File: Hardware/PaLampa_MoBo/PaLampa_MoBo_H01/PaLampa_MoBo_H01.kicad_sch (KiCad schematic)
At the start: 47 parts, among them J1 Conn_01x03_Male, J9 Conn_01x05_Male, Q1 2N7002, Q4 2N7002, SW1 SW_SPST, SW2 SW_SPST, SW3 SW_SPST, U1 ESP32-WROOM-32D, U2 DS18B20, U3 OLED_I2C

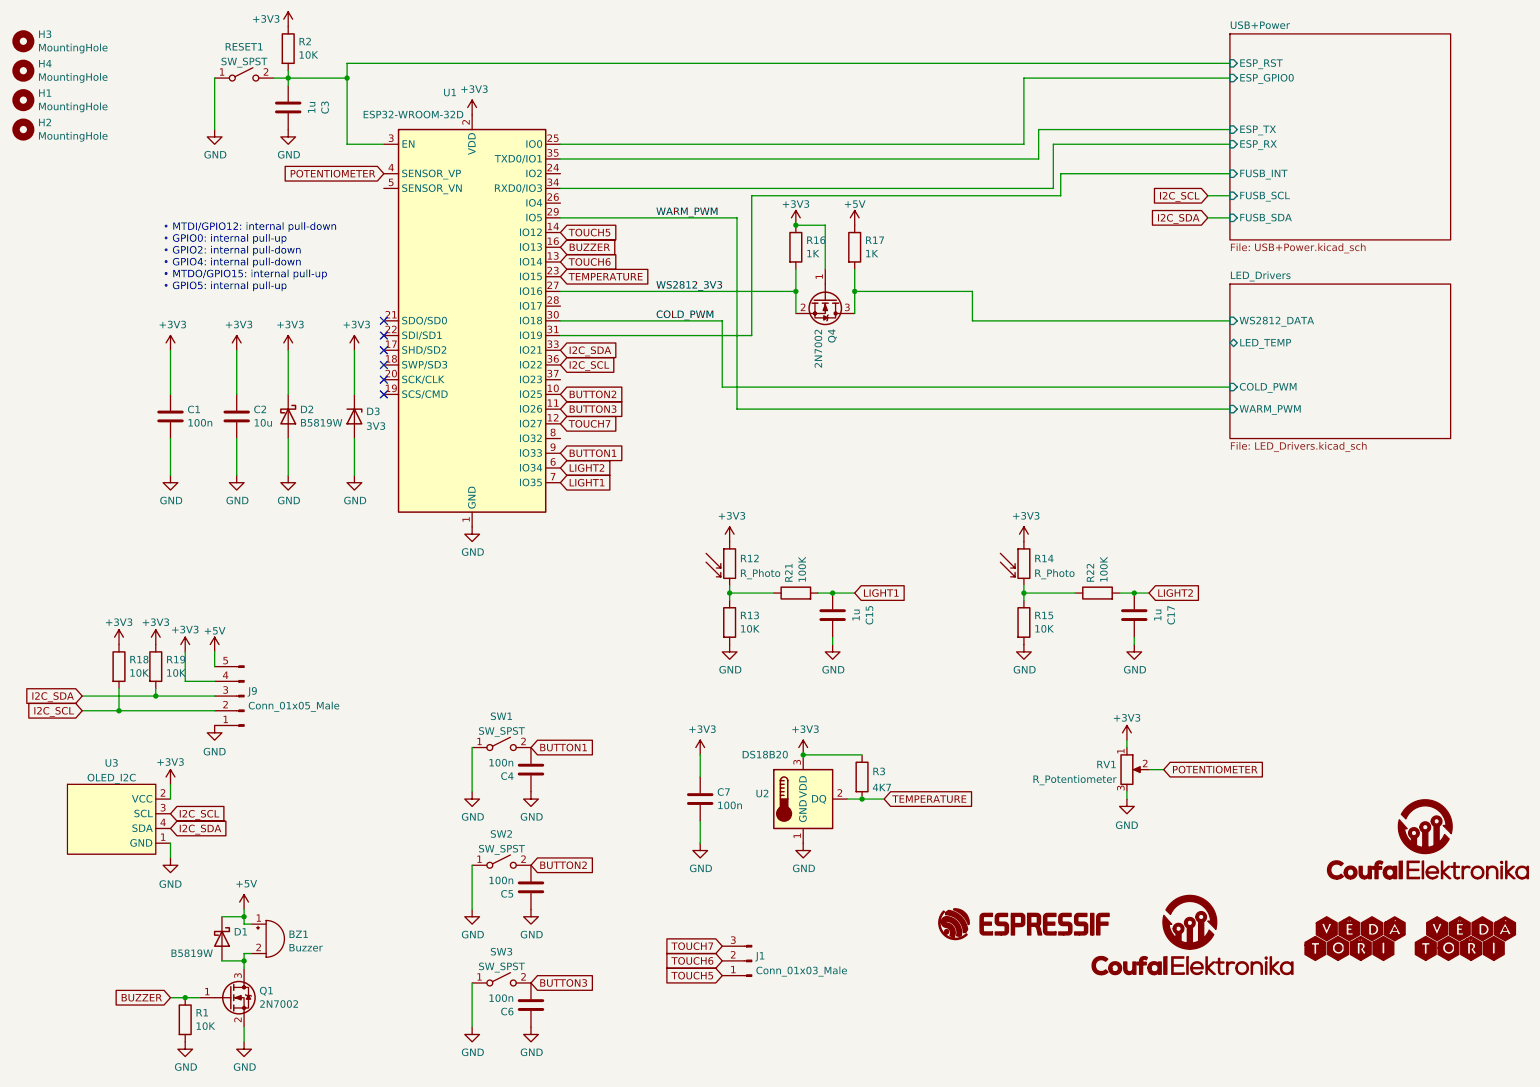
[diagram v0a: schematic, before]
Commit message: H01 update
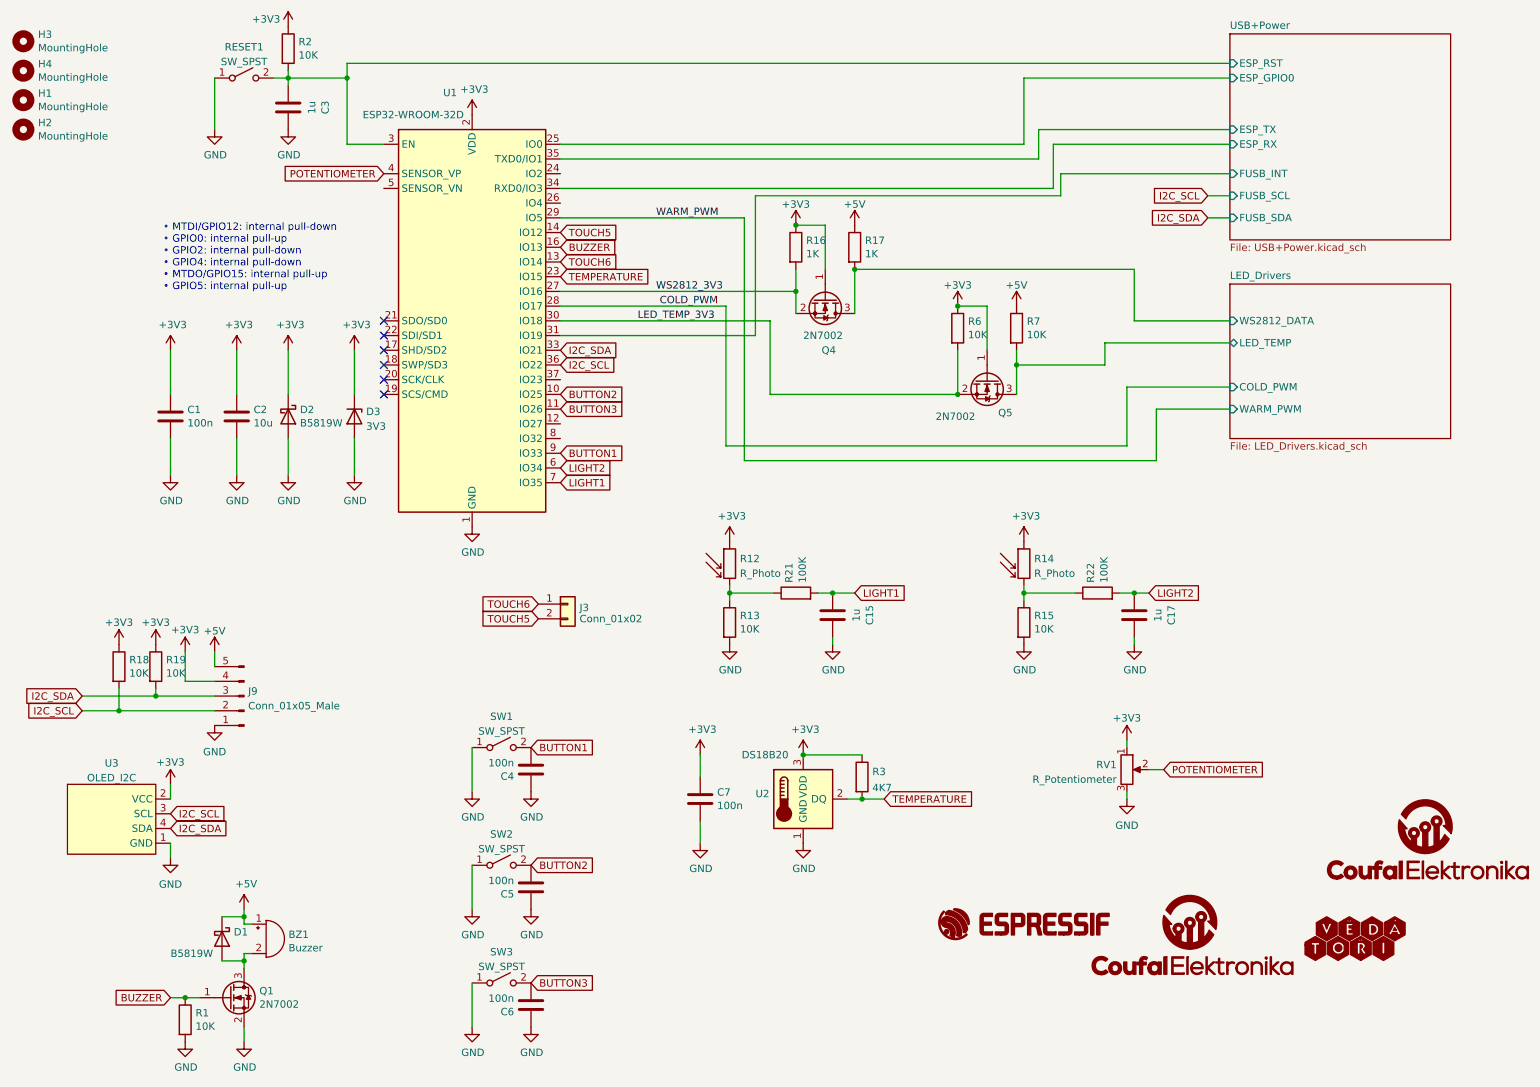
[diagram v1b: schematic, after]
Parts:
- removed G3: Vedatori_logo, PaLampa_Library:VedatoriNew_40x5,7mm, symbol Time-O-Mat_Library:Vedatori_logo
- removed J1: Conn_01x03_Male, Connector_PinHeader_2.54mm:PinHeader_1x03_P2.54mm_Vertical, symbol Connector:Conn_01x03_Male
- added J3: Conn_01x02, Connector_JST:JST_XH_B2B-XH-A_1x02_P2.50mm_Vertical, symbol Connector_Generic:Conn_01x02
- added Q5: 2N7002, Package_TO_SOT_SMD:SOT-23, symbol Transistor_FET:2N7002
- added R6, R7: 10K, Resistor_SMD:R_0603_1608Metric, symbol Device:R
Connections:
- net +3V3: now also Q5.1 (G), R6.1
- net +5V: now also R7.1
- net COLD_PWM: now also U1.28 (IO17); no longer U1.30 (IO18)
- net LED_Drivers/LED_TEMP: now also Q5.3 (D), R7.2
- net TOUCH5: now also J3.2 (Pin_2)
- net TOUCH6: now also J3.1 (Pin_1)
- net TOUCH7: no longer names the net of U1.12 (IO27)
- new net LED_TEMP_3V3: Q5.2 (S), R6.2, U1.30 (IO18)
